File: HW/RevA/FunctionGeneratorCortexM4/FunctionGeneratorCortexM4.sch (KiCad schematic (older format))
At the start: 5 parts

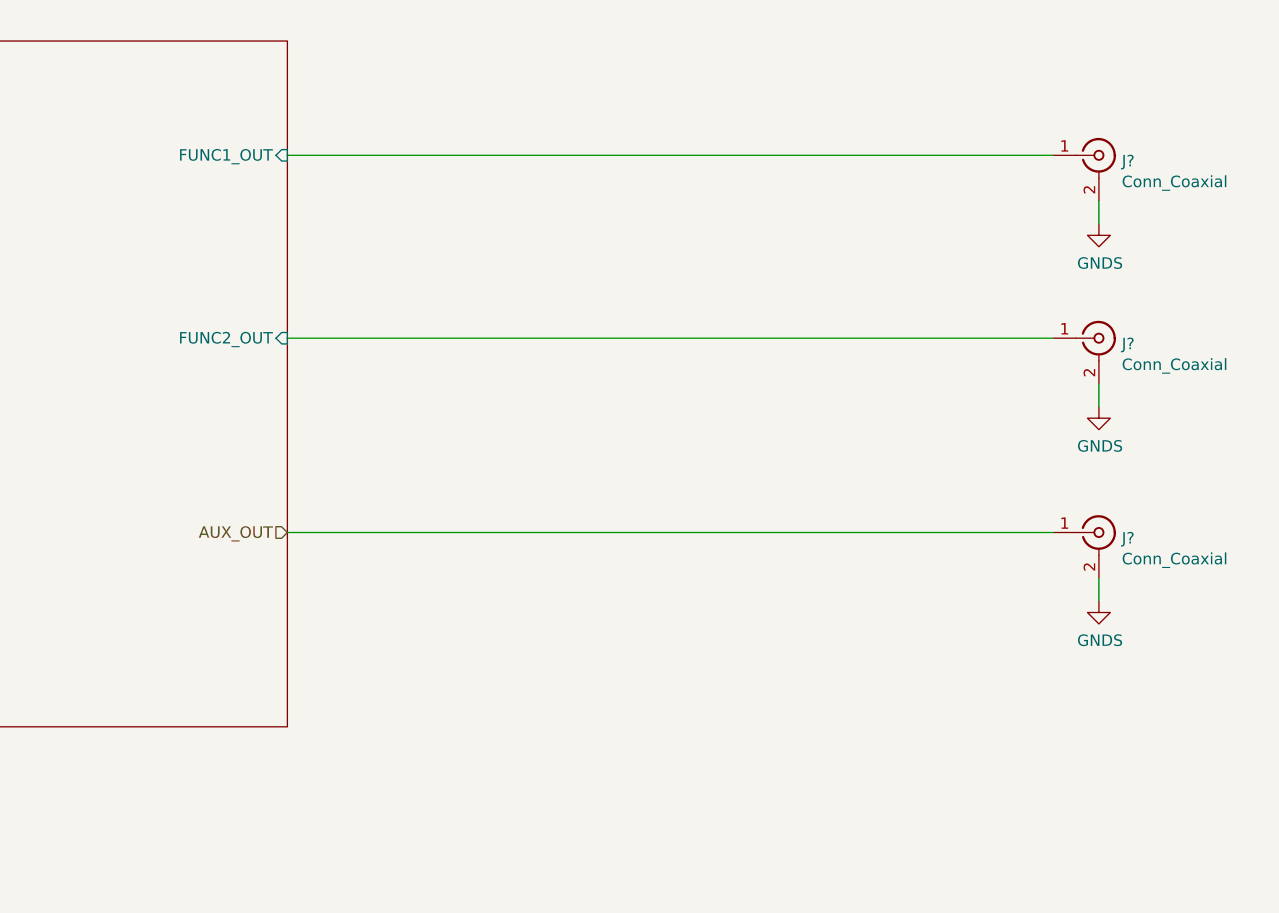
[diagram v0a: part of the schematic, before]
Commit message: hw update
- Added MCU section
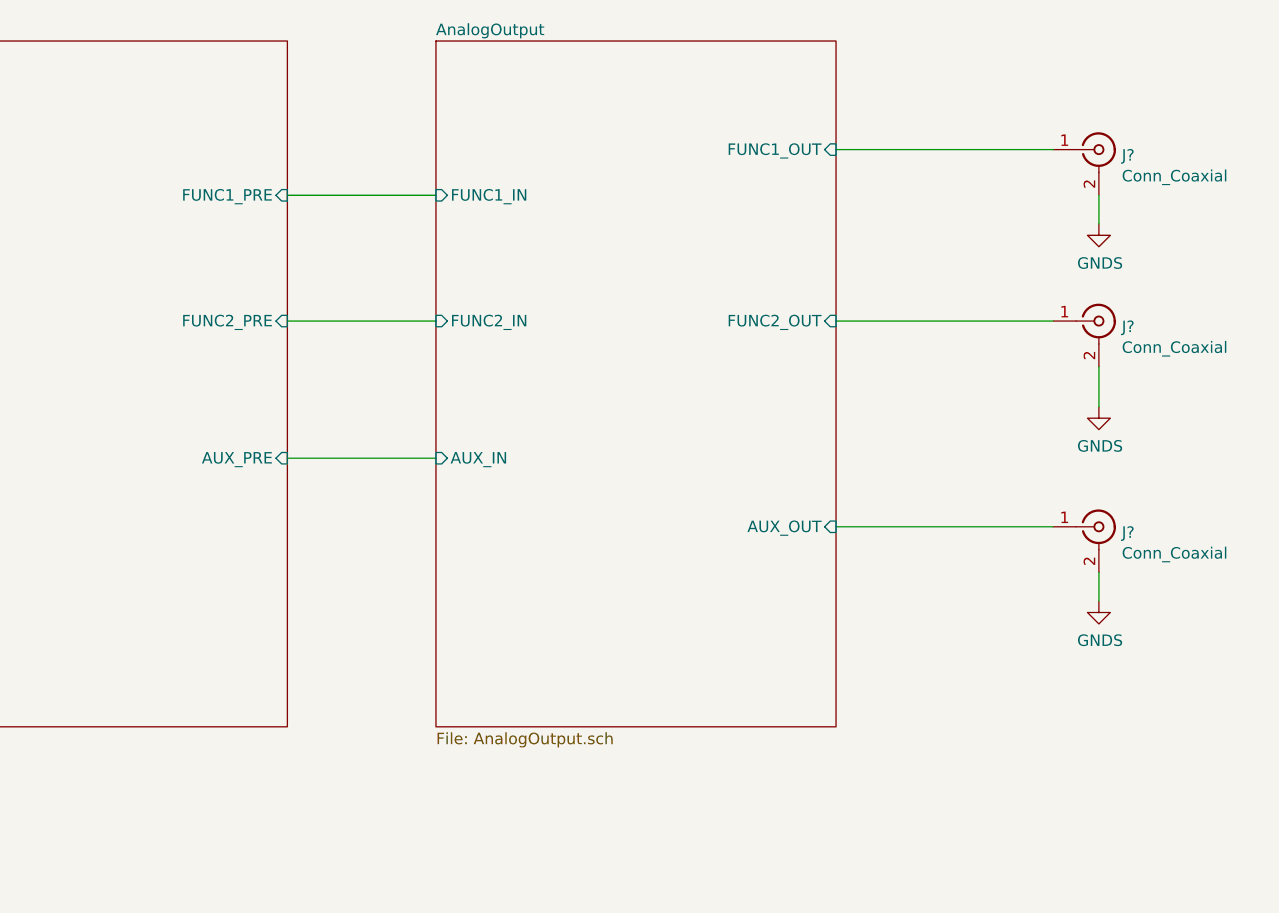
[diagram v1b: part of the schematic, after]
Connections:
- net AUX_OUT renamed AnalogOutput/AUX_OUT
- net MCU/FUNC1_OUT renamed AnalogOutput/FUNC1_OUT
- net MCU/FUNC2_OUT renamed AnalogOutput/FUNC2_OUT
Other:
- moved on the sheet: J?
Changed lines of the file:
@@
 $Descr A4 11693 8268
 encoding utf-8
-Sheet 1 3
+Sheet 1 4
 Title ""
 Date ""
@@
 F1 "MCU.sch" 50
 F2 "TRIG_IN" I L 3700 2150 50
-F3 "FUNC1_OUT" I R 6350 2000 50
-F4 "FUNC2_OUT" I R 6350 2800 50
+F3 "FUNC1_PRE" I R 6350 2175 50
+F4 "FUNC2_PRE" I R 6350 2725 50
+F5 "AUX_PRE" I R 6350 3325 50
 $EndSheet
 $Sheet
@@
 L Connector:Conn_Coaxial J?
 U 1 1 5E6C10C9
-P 9900 2000
-F 0 "J?" H 10000 1975 50  0000 L CNN
-F 1 "Conn_Coaxial" H 10000 1884 50  0000 L CNN
-F 2 "" H 9900 2000 50  0001 C CNN
-F 3 " ~" H 9900 2000 50  0001 C CNN
-	1    9900 2000
+P 9900 1975
+F 0 "J?" H 10000 1950 50  0000 L CNN
+F 1 "Conn_Coaxial" H 10000 1859 50  0000 L CNN
+F 2 "" H 9900 1975 50  0001 C CNN
+F 3 " ~" H 9900 1975 50  0001 C CNN
+	1    9900 1975
 	1    0    0    -1
 $EndComp
@@
 L Connector:Conn_Coaxial J?
 U 1 1 5E6C23B8
-P 9900 2800
-F 0 "J?" H 10000 2775 50  0000 L CNN
-F 1 "Conn_Coaxial" H 10000 2684 50  0000 L CNN
-F 2 "" H 9900 2800 50  0001 C CNN
-F 3 " ~" H 9900 2800 50  0001 C CNN
-	1    9900 2800
+P 9900 2725
+F 0 "J?" H 10000 2700 50  0000 L CNN
+F 1 "Conn_Coaxial" H 10000 2609 50  0000 L CNN
+F 2 "" H 9900 2725 50  0001 C CNN
+F 3 " ~" H 9900 2725 50  0001 C CNN
+	1    9900 2725
 	1    0    0    -1
 $EndComp
 Wire Wire Line
-	9900 2200 9900 2300
+	9900 2175 9900 2300
 $Comp
 L power:GNDS #PWR?
@@
 $EndComp
 Wire Wire Line
-	9900 3000 9900 3100
+	9900 2925 9900 3100
 $Comp
 L power:GNDS #PWR?
@@
 Wire Wire Line
 	3700 2150 1800 2150
-Wire Wire Line
-	6350 2000 9700 2000
-Wire Wire Line
-	6350 2800 9700 2800
 $Comp
 L Connector:Conn_Coaxial J?
 U 1 1 5E6DBAC5
-P 9900 3650
-F 0 "J?" H 10000 3625 50  0000 L CNN
-F 1 "Conn_Coaxial" H 10000 3534 50  0000 L CNN
-F 2 "" H 9900 3650 50  0001 C CNN
-F 3 " ~" H 9900 3650 50  0001 C CNN
-	1    9900 3650
+P 9900 3625
+F 0 "J?" H 10000 3600 50  0000 L CNN
+F 1 "Conn_Coaxial" H 10000 3509 50  0000 L CNN
+F 2 "" H 9900 3625 50  0001 C CNN
+F 3 " ~" H 9900 3625 50  0001 C CNN
+	1    9900 3625
 	1    0    0    -1
 $EndComp
 Wire Wire Line
-	9900 3850 9900 3950
+	9900 3825 9900 3950
 $Comp
 L power:GNDS #PWR?
@@
 	1    0    0    -1
 $EndComp
+$Sheet
+S 7000 1500 1750 3000
+U 5EBB9B06
+F0 "AnalogOutput" 50
+F1 "AnalogOutput.sch" 50
+F2 "AUX_IN" I L 7000 3325 50
+F3 "FUNC1_IN" I L 7000 2175 50
+F4 "FUNC2_IN" I L 7000 2725 50
+F5 "AUX_OUT" I R 8750 3625 50
+F6 "FUNC1_OUT" I R 8750 1975 50
+F7 "FUNC2_OUT" I R 8750 2725 50
+$EndSheet
 Wire Wire Line
-	6350 3650 9700 3650
-Text HLabel 6350 3650 0    50   Input ~ 0
-AUX_OUT
+	7000 2175 6350 2175
+Wire Wire Line
+	6350 2725 7000 2725
+Wire Wire Line
+	7000 3325 6350 3325
+Wire Wire Line
+	8750 3625 9700 3625
+Wire Wire Line
+	8750 2725 9700 2725
+Wire Wire Line
+	8750 1975 9700 1975
 $EndSCHEMATC
